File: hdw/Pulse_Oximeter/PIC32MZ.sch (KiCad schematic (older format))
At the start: 1 part

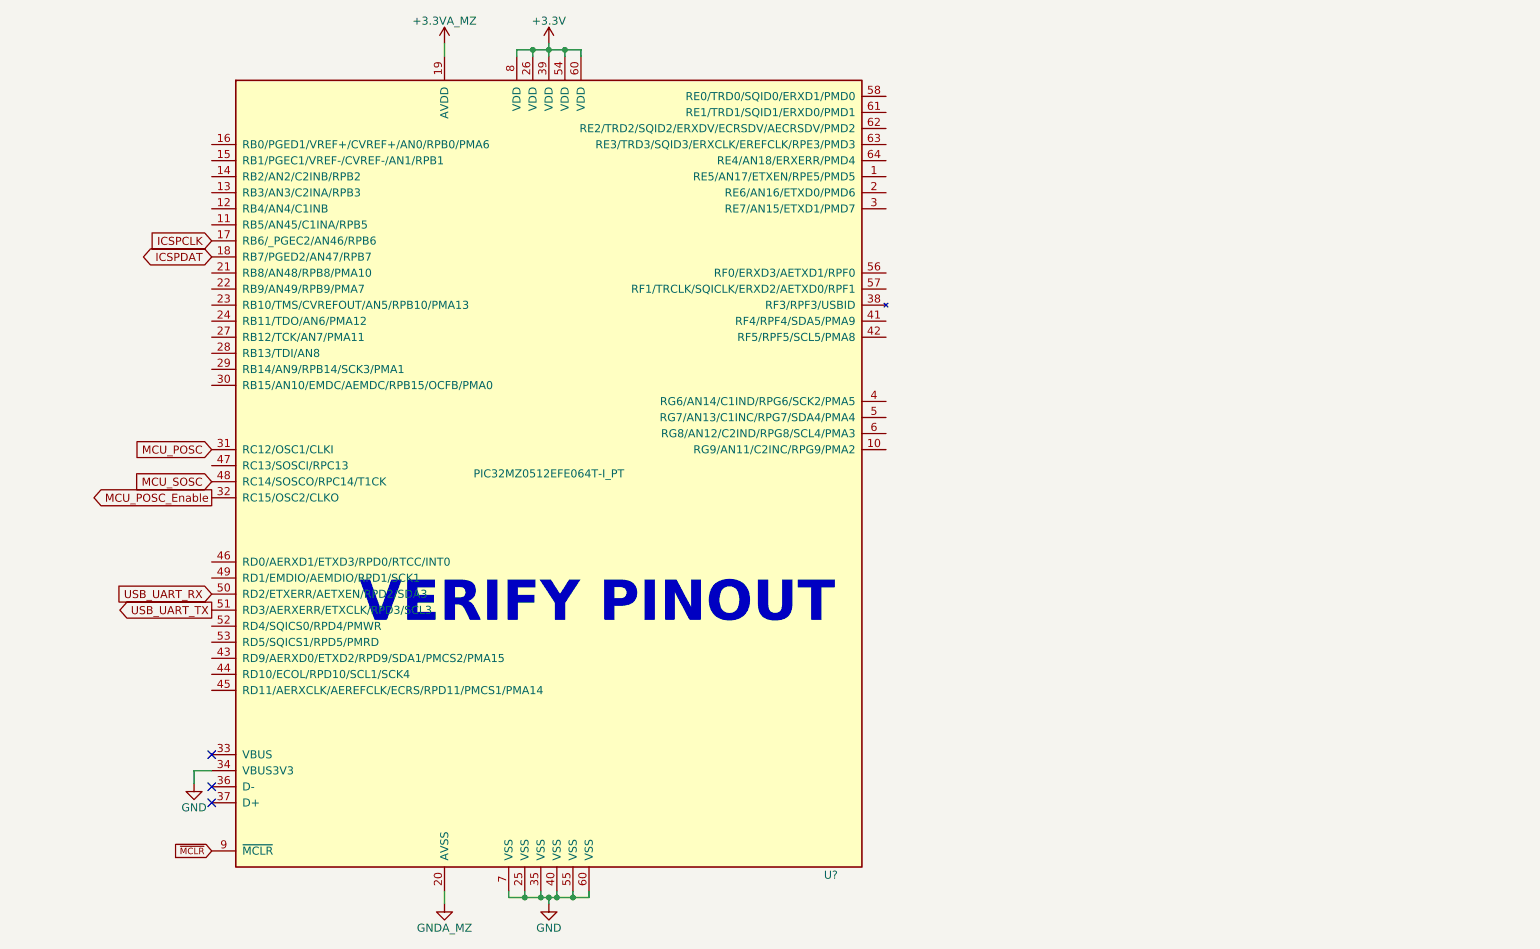
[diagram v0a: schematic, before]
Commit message: Added display circuits
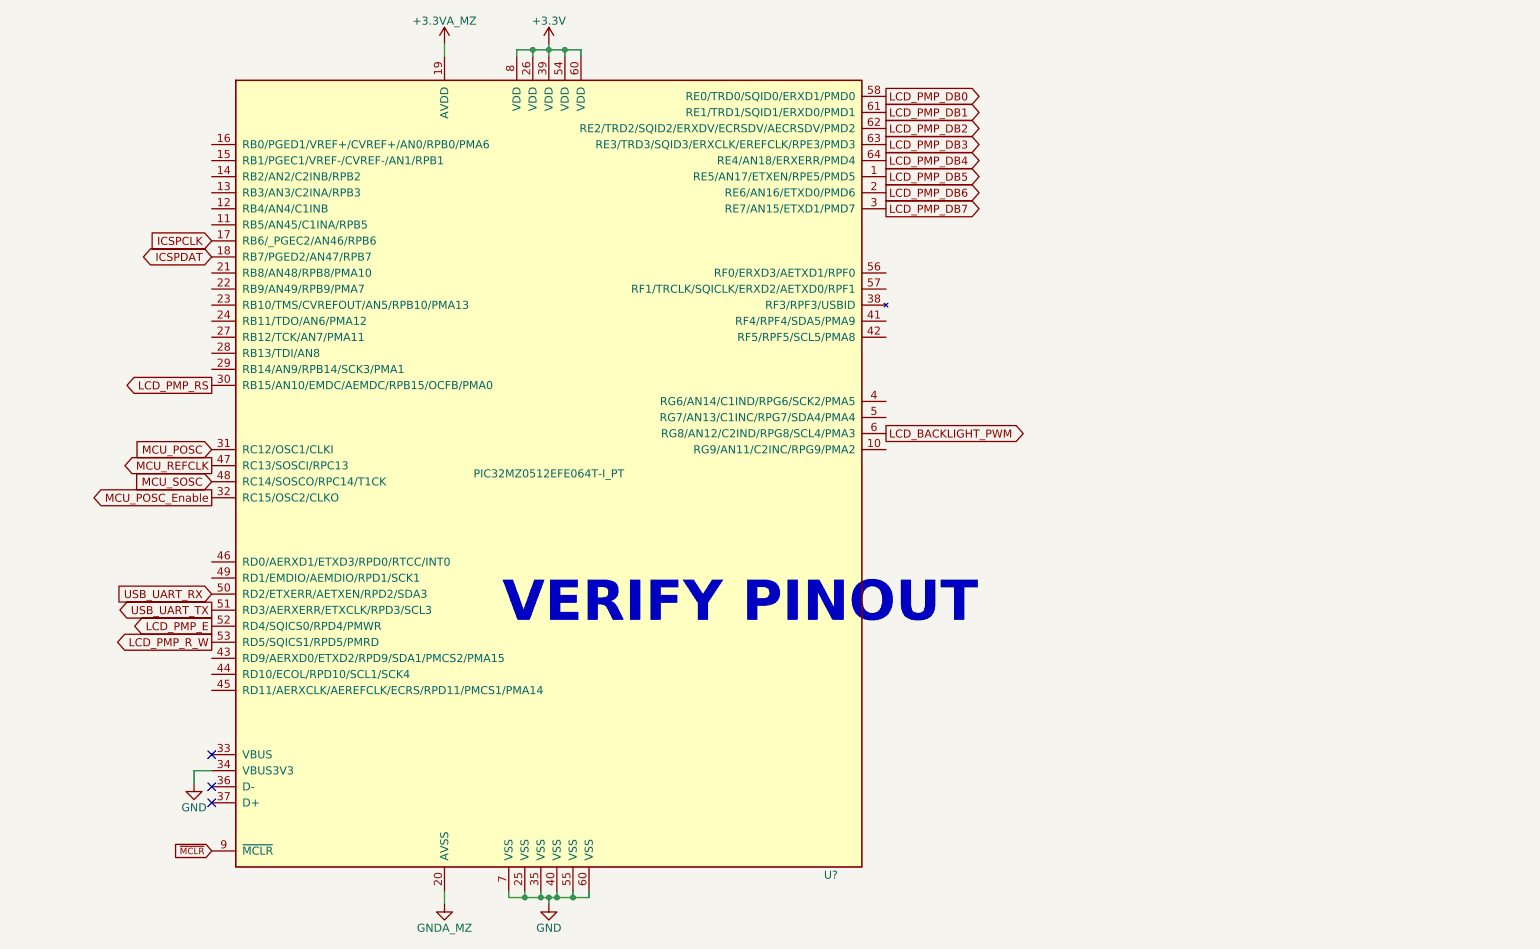
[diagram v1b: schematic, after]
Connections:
- net LCD_PMP_DB5: now reaches U?.1 (RE5/AN17/ETXEN/RPE5/PMD5)
- net LCD_PMP_DB6: now reaches U?.2 (RE6/AN16/ETXD0/PMD6)
- net LCD_PMP_DB7: now reaches U?.3 (RE7/AN15/ETXD1/PMD7)
- net LCD_PMP_RS: now reaches U?.30 (RB15/AN10/EMDC/AEMDC/RPB15/OCFB/PMA0)
- net MCU_REFCLK: now reaches U?.47 (RC13/SOSCI/RPC13)
- net LCD_PMP_E: now reaches U?.52 (RD4/SQICS0/RPD4/PMWR)
- net LCD_PMP_R_W: now reaches U?.53 (RD5/SQICS1/RPD5/PMRD)
- net LCD_PMP_DB0: now reaches U?.58 (RE0/TRD0/SQID0/ERXD1/PMD0)
- net LCD_BACKLIGHT_PWM: now reaches U?.6 (RG8/AN12/C2IND/RPG8/SCL4/PMA3)
- net LCD_PMP_DB1: now reaches U?.61 (RE1/TRD1/SQID1/ERXD0/PMD1)
- net LCD_PMP_DB2: now reaches U?.62 (RE2/TRD2/SQID2/ERXDV/ECRSDV/AECRSDV/PMD2)
- net LCD_PMP_DB3: now reaches U?.63 (RE3/TRD3/SQID3/ERXCLK/EREFCLK/RPE3/PMD3)
- net LCD_PMP_DB4: now reaches U?.64 (RE4/AN18/ERXERR/PMD4)
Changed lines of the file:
@@
 EESchema Schematic File Version 4
+LIBS:Pulse_Oximeter-cache
 EELAYER 30 0
 EELAYER END
@@
 NoConn ~ 3360 5510
 NoConn ~ 3360 5610
-Text Notes 4280 4510 0    250  ~ 50
+Text Notes 5170 4510 0    250  ~ 50
 VERIFY PINOUT
 $Comp
@@
 	1    0    0    -1
 $EndComp
+Text GLabel 7560 3310 2    50   Output ~ 0
+LCD_BACKLIGHT_PWM
+Text GLabel 3360 3010 0    50   Output ~ 0
+LCD_PMP_RS
+Text GLabel 3360 4610 0    50   Output ~ 0
+LCD_PMP_R_W
+Text GLabel 3360 4510 0    50   Output ~ 0
+LCD_PMP_E
+Text GLabel 7560 1210 2    50   Output ~ 0
+LCD_PMP_DB0
+Text GLabel 7560 1310 2    50   Output ~ 0
+LCD_PMP_DB1
+Text GLabel 7560 1410 2    50   Output ~ 0
+LCD_PMP_DB2
+Text GLabel 7560 1510 2    50   Output ~ 0
+LCD_PMP_DB3
+Text GLabel 7560 1610 2    50   Output ~ 0
+LCD_PMP_DB4
+Text GLabel 7560 1710 2    50   Output ~ 0
+LCD_PMP_DB5
+Text GLabel 7560 1810 2    50   Output ~ 0
+LCD_PMP_DB6
+Text GLabel 7560 1910 2    50   Output ~ 0
+LCD_PMP_DB7
+Text GLabel 3360 3510 0    50   Output ~ 0
+MCU_REFCLK
 $EndSCHEMATC

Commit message: few sch additions
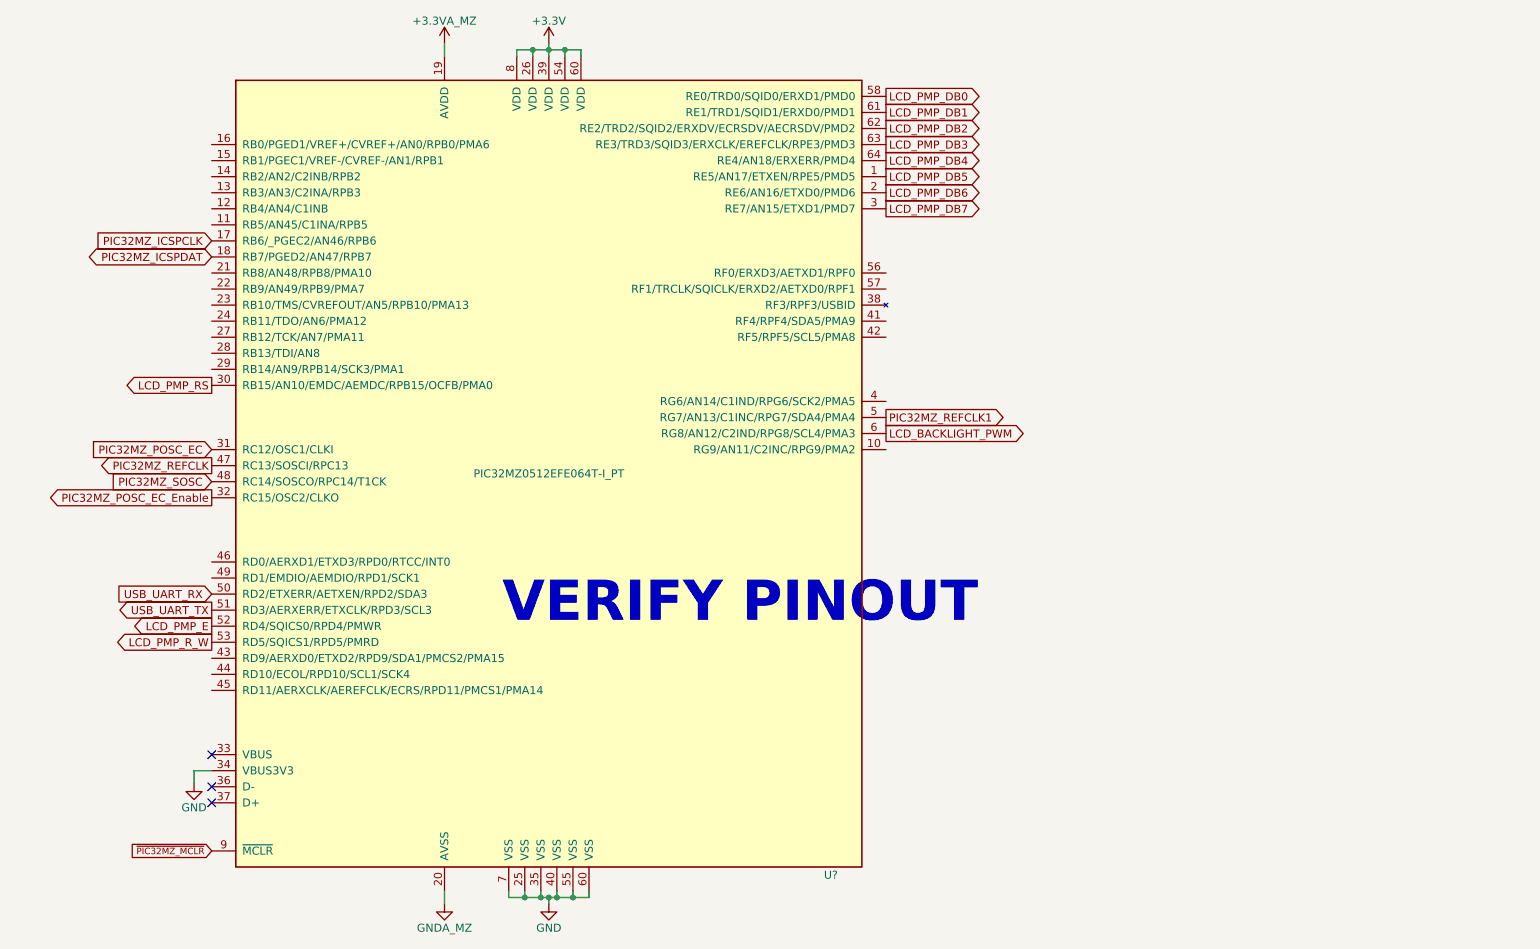
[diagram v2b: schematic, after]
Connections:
- net PIC32MZ_REFCLK1: now reaches U?.5 (RG7/AN13/C1INC/RPG7/SDA4/PMA4)
- net ICSPCLK renamed PIC32MZ_ICSPCLK
- net ICSPDAT renamed PIC32MZ_ICSPDAT
- net MCU_POSC renamed PIC32MZ_POSC_EC
- net MCU_POSC_Enable renamed PIC32MZ_POSC_EC_Enable
- net MCU_REFCLK renamed PIC32MZ_REFCLK
- net MCU_SOSC renamed PIC32MZ_SOSC
- net ~MCLR renamed ~PIC32MZ_MCLR
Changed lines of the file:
@@
 	4810 880  4810 960
 Text GLabel 3360 5910 0    40   Input ~ 0
-~MCLR
+~PIC32MZ_MCLR
 $Comp
 L power:GND #PWR?
@@
 	3250 5410 3360 5410
 Text GLabel 3360 3410 0    50   Input ~ 0
-MCU_POSC
+PIC32MZ_POSC_EC
 Text GLabel 3360 3610 0    50   Input ~ 0
-MCU_SOSC
+PIC32MZ_SOSC
 Text GLabel 3360 2210 0    50   BiDi ~ 0
-ICSPDAT
+PIC32MZ_ICSPDAT
 Text GLabel 3360 2110 0    50   Input ~ 0
-ICSPCLK
+PIC32MZ_ICSPCLK
 Text GLabel 3360 3710 0    50   Output ~ 0
-MCU_POSC_Enable
+PIC32MZ_POSC_EC_Enable
 Text GLabel 3360 4310 0    50   Input ~ 0
 USB_UART_RX
@@
 LCD_PMP_DB7
 Text GLabel 3360 3510 0    50   Output ~ 0
-MCU_REFCLK
+PIC32MZ_REFCLK
+Text GLabel 7560 3210 2    50   Output ~ 0
+PIC32MZ_REFCLK1
 $EndSCHEMATC

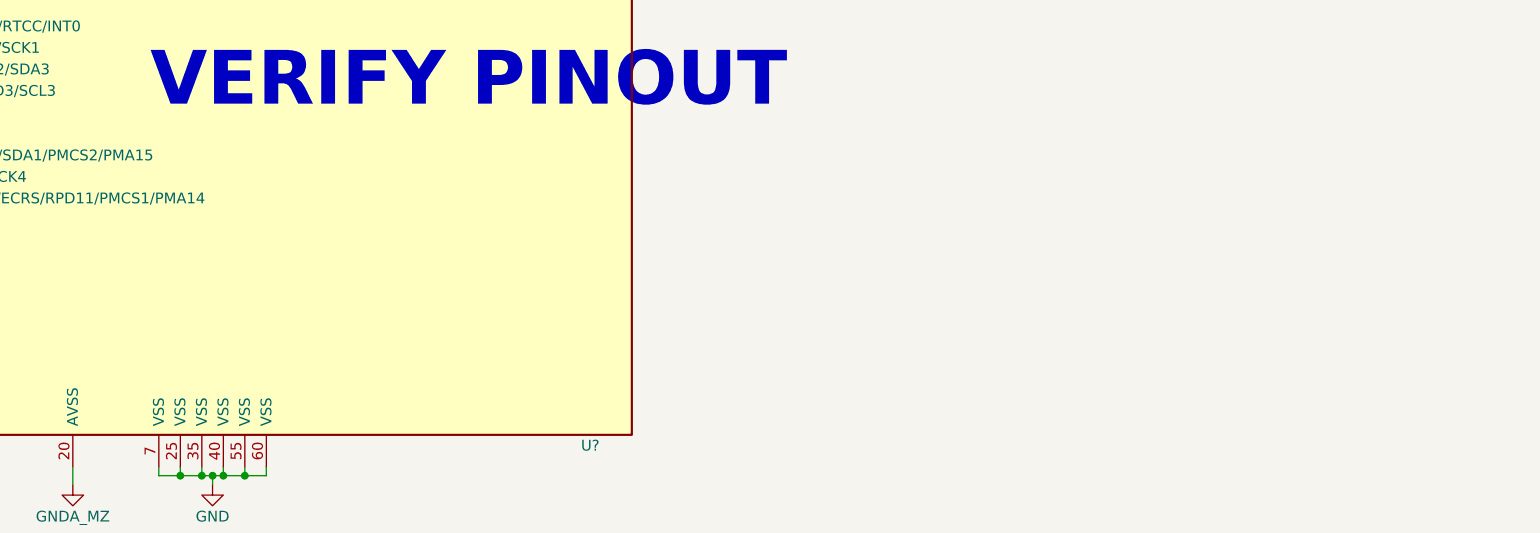
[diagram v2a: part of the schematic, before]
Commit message: More sch work
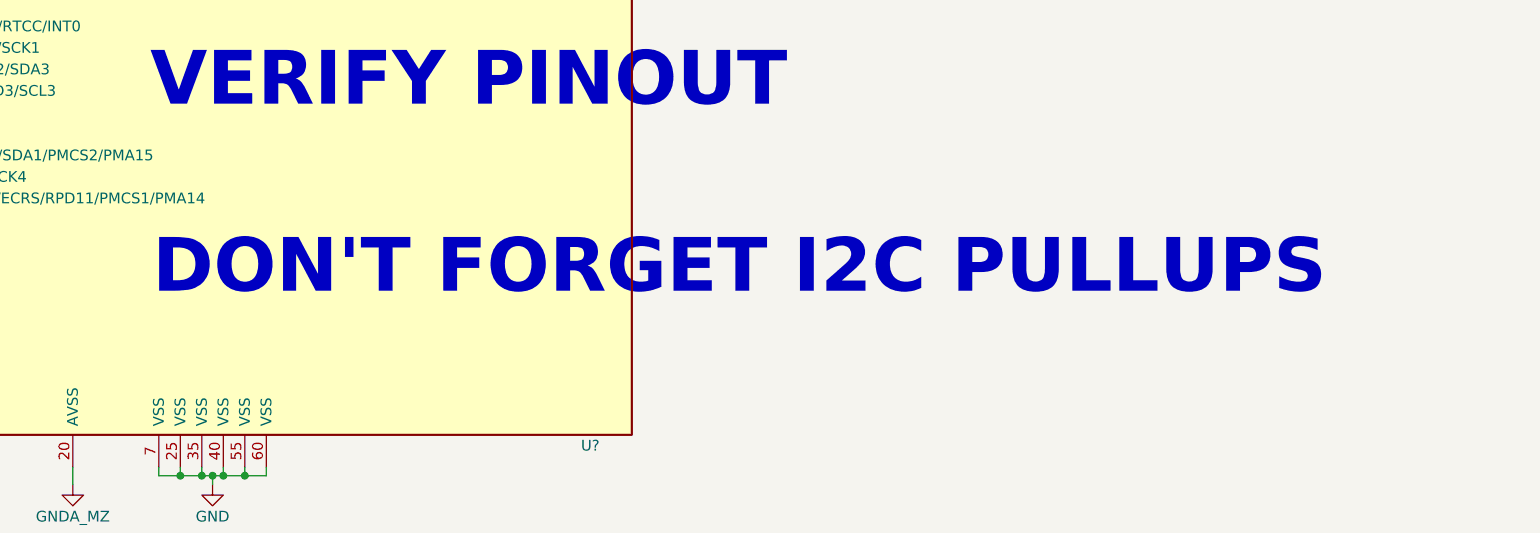
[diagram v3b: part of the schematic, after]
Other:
- note added: "DON'T FORGET I2C PULLUPS"
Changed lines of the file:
@@
 Text GLabel 7560 3210 2    50   Output ~ 0
 PIC32MZ_REFCLK1
+Text Notes 5180 5380 0    250  ~ 50
+DON'T FORGET I2C PULLUPS
 $EndSCHEMATC
